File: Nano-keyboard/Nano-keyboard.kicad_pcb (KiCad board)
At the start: 2 copper layers, 120.1 x 80.2 mm, 39 parts, among them U1 QBC847BL, U2 ESP32-WROOM-32, U3 QBC847BL, U4 QBC847BL, U5 EN12-HN22AF25, U6 EN12-HN22AF25, U7 TP4050

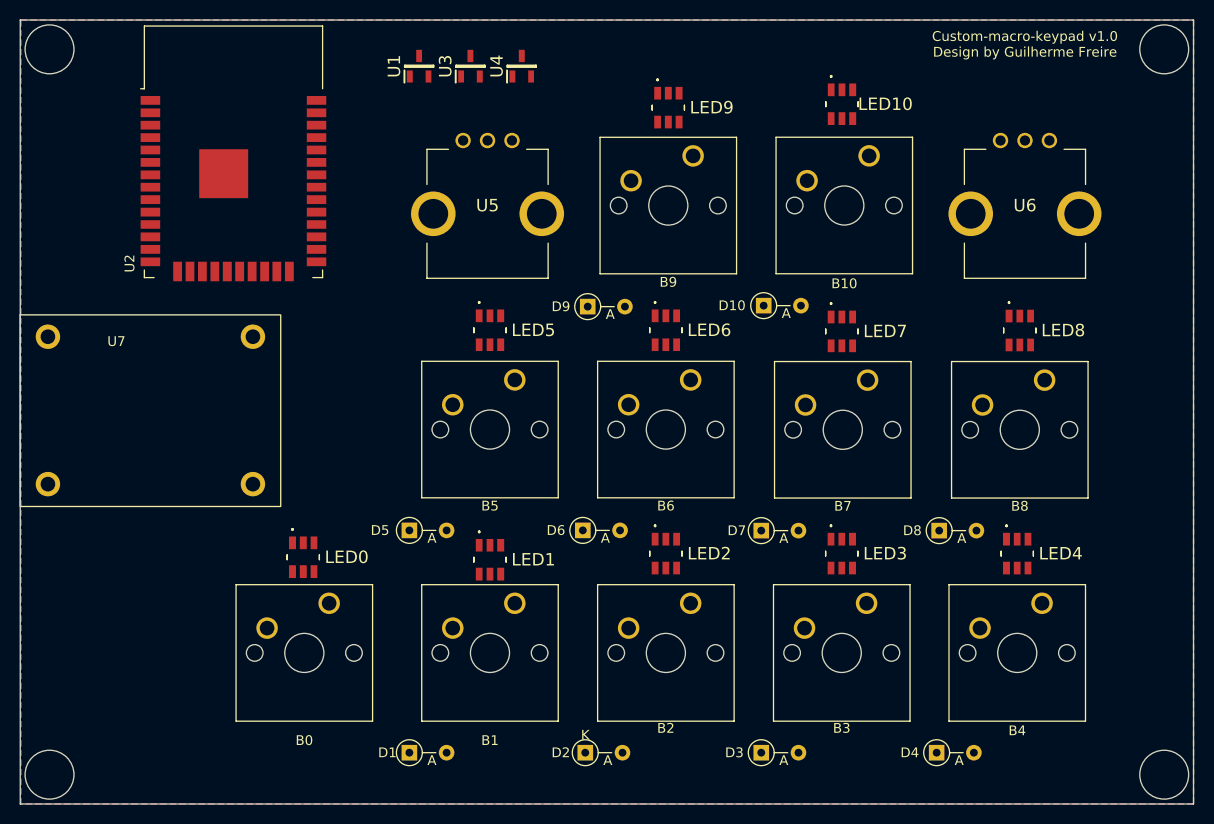
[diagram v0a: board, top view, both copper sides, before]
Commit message: Minor changes
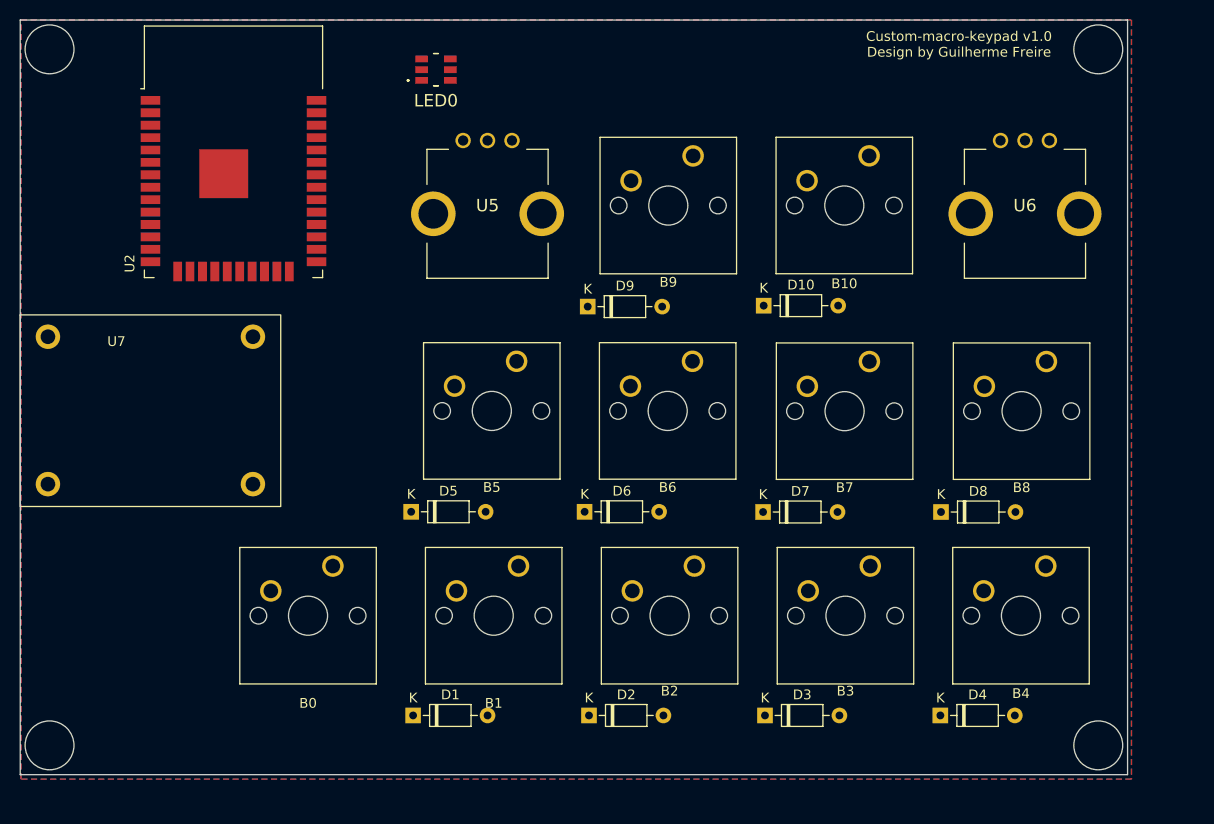
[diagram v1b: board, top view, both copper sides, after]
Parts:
- removed LED1, LED10, LED2, LED3, LED4, LED5, LED6, LED7, LED8, LED9: LRTBGVSR-U4V2-JW+A6BB-D8+S2U2-7Z-20-S, lib:LRTBGVSRU4V2JWA6BBD8S2U27Z20S
- removed U1, U3, U4: QBC847BL, lib:SOT96P237X111-3N
- D1, D10, D2, D3, D4, D5, D6, D7, D8, D9: footprint Diode_THT:D_DO-35_SOD27_P3.81mm_Vertical_AnodeUp -> Diode_THT:D_DO-35_SOD27_P7.62mm_Horizontal
- moved LED0 51.7 mm to (109.2, 69.8), turned to 90 degrees
- moved D1 3.83 mm to (106.9, 135.9)
- moved D2 3.83 mm to (124.9, 135.9)
- moved D3 3.83 mm to (142.9, 135.9)
- moved D4 3.83 mm to (160.8, 135.9)
- moved B0 3.83 mm to (98.7, 120.7)
- moved B1 3.83 mm to (117.7, 120.7)
- moved B2 3.83 mm to (135.7, 120.7)
- moved B3 3.83 mm to (153.7, 120.7)
- moved B4 3.83 mm to (171.6, 120.7)
- moved B6 1.91 mm to (135.5, 99.7)
- moved D5 1.91 mm to (106.7, 115.1)
- moved D6 1.91 mm to (124.4, 115.1)
- moved D7 1.91 mm to (142.7, 115.1)
- moved D8 1.91 mm to (160.9, 115.1)
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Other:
- board size 120.1 x 80.2 mm -> 113.3 x 77.2 mm
